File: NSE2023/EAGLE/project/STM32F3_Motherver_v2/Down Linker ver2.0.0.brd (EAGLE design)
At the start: 35.5 x 45.4 mm, 27 parts

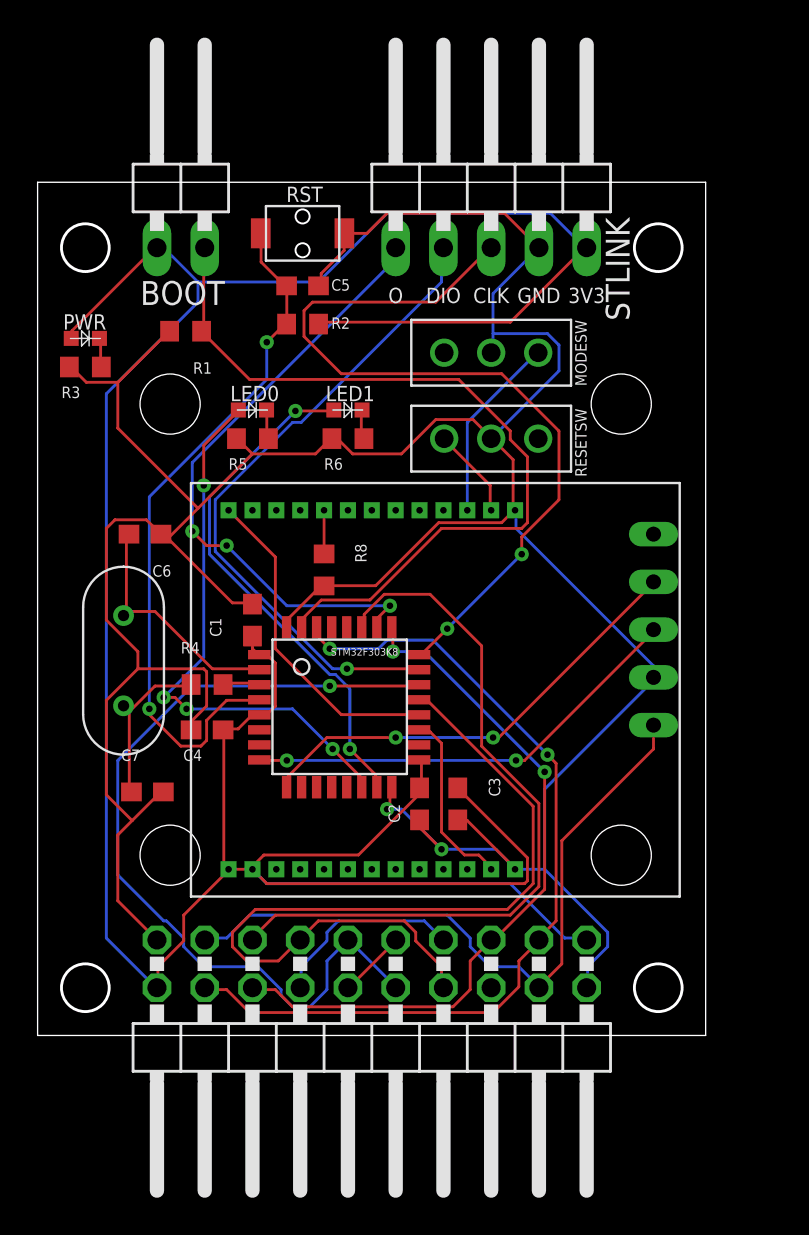
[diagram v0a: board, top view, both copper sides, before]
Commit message: create final board NSE2023
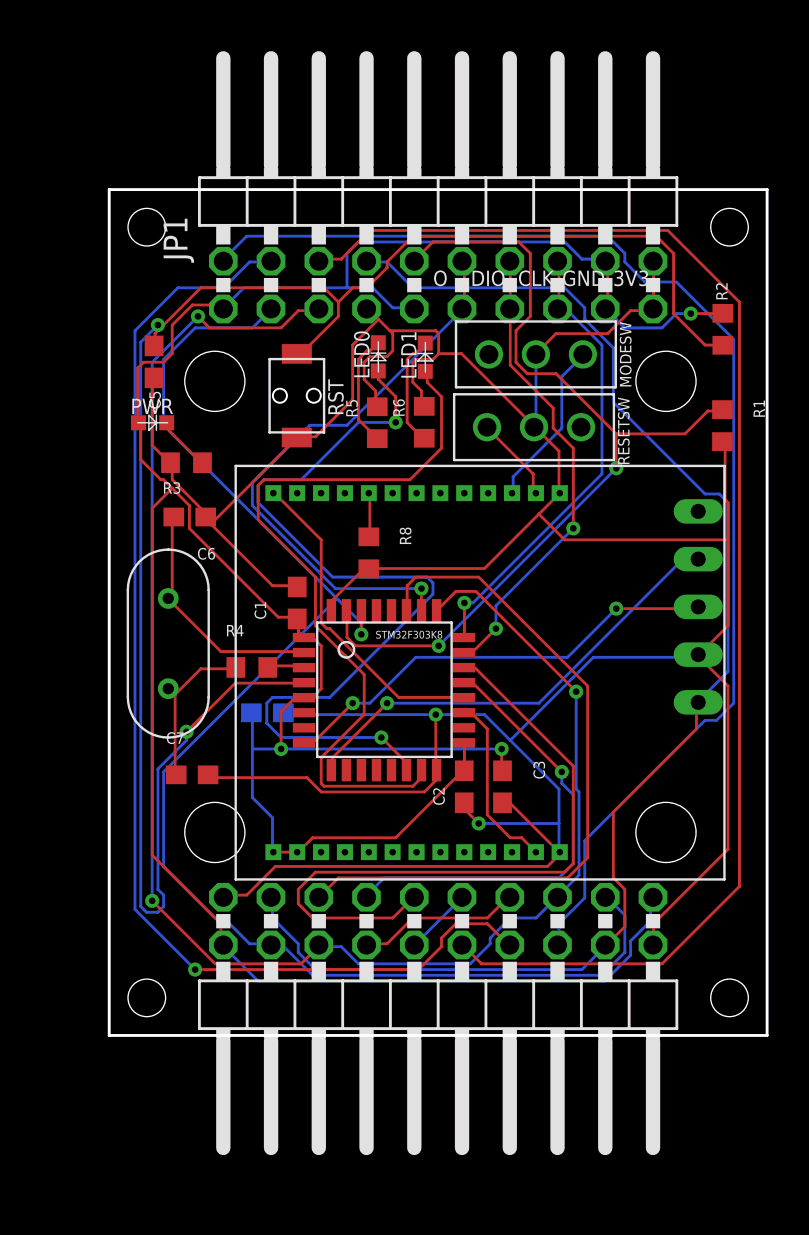
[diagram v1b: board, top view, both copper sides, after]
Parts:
- removed BOOT: (no value), pinhead:1X02/90
- removed STLINK: (no value), pinhead:1X05/90
- added JP1: (no value), pinhead:2X10/90
- added U$4: F.T.E.LOGO, logo:LOGO
- moved R1 29.0 mm to (32.6, 32.4), turned to 270 degrees
- moved R2 22.4 mm to (32.6, 37.6), turned to 90 degrees
- moved C5 8.87 mm to (2.39, 35.8), turned to 270 degrees
- moved RST 8.64 mm to (9.98, 34.0), turned to 0 degrees
- moved R3 7.41 mm to (4.11, 30.5)
- moved LED0 7.27 mm to (14.3, 36.1), turned to 90 degrees
- moved R5 6.69 mm to (14.3, 32.6), turned to 270 degrees
- moved PWR 5.74 mm to (2.31, 32.6)
- moved LED1 4.98 mm to (16.8, 36.1), turned to 90 degrees
- moved JP3 4.20 mm to (17.5, 1.00)
- moved R6 4.15 mm to (16.8, 32.6), turned to 270 degrees
- moved C4 3.33 mm to (8.41, 17.2), flipped to the bottom
- moved U$2 2.67 mm to (17.6, 22.8)
- moved R8 2.55 mm to (13.8, 25.7)
- moved U$1 2.55 mm to (11.0, 14.1)
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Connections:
- new net FPRAW: JP1.6, JP3.10
- new net SW: JP1.4, JP3.8
- net +3V3: now also JP1.1, JP1.17, JP1.18, JP1.9; no longer BOOT.1, STLINK.5
- net +5V: now also JP1.8
- net BIT1: no longer JP3.10
- net BIT2: no longer JP3.8
- net BOOT0: now also JP1.10; no longer BOOT.2
- net GND: now also JP1.19, JP1.20, JP1.7; no longer STLINK.4
- net PWM: now also JP1.2
- net SCL: now also JP1.5
- net SDA: now also JP1.3
- net SWCLK: now also JP1.15, JP1.16; no longer STLINK.3
- net SWDIO: now also JP1.13, JP1.14; no longer STLINK.2
- net SWO: now also JP1.11, JP1.12; no longer STLINK.1
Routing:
- net FPRAW: track 0.00 -> 72.6 mm
- net PWM: track 0.00 -> 66.8 mm
- net SW: track 0.00 -> 62.5 mm, vias 0 -> 1
- net NRST: track 37.5 -> 92.5 mm
- net SCL: track 37.8 -> 86.2 mm, vias 2 -> 3
- net +5V: track 36.7 -> 74.2 mm
- net SDA: track 46.9 -> 76.1 mm, vias 2 -> 1
- net BIT2: track 45.2 -> 24.1 mm, vias 0 -> 1
- net GND: track 183.3 -> 202.8 mm
- net SWCLK: track 43.4 -> 24.7 mm, vias 2 -> 1
- net LED0: track 29.7 -> 45.4 mm, vias 4 -> 2
- net LED1: track 27.8 -> 40.1 mm, vias 2 -> 0
- net SWDIO: track 35.0 -> 24.9 mm, vias 1 -> 2
- net BIT1: track 45.4 -> 36.1 mm, vias 1 -> 0
- net +3V3: track 167.2 -> 159.5 mm, vias 0 -> 3
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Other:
- board size 35.5 x 45.4 mm -> 35 x 45 mm

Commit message: www
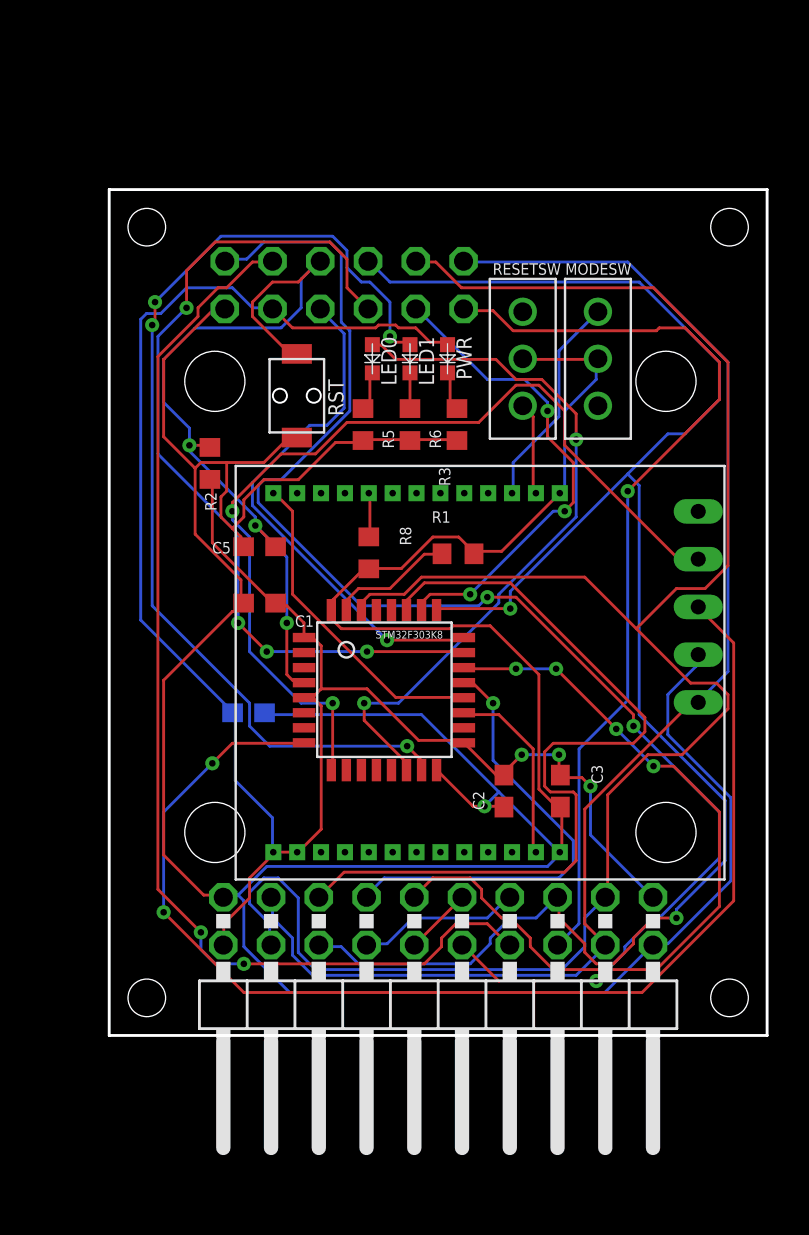
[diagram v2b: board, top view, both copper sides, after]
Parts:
- removed C6, C7: 30pF, rcl:C1608
- removed CRY1: (no value), Crystal:CRYSTAL
- removed JP1: (no value), pinhead:2X10/90
- removed R4: DNF, rcl:R0603
- removed U$4: F.T.E.LOGO, logo:LOGO
- added JP2: (no value), pinhead:2X06/90
- moved R2 28.2 mm to (5.36, 30.4), turned to 270 degrees
- moved PWR 16.1 mm to (18.0, 36.0), turned to 270 degrees
- moved R1 15.6 mm to (18.6, 25.6), turned to 0 degrees
- moved R3 14.5 mm to (18.5, 32.5), turned to 90 degrees
- moved C5 11.3 mm to (8.00, 26.0), turned to 180 degrees
- moved RESETSW 3.69 mm to (22.0, 36.0), turned to 270 degrees
- moved MODESW 3.31 mm to (26.0, 36.0), turned to 90 degrees
- moved C3 3.09 mm to (24.0, 13.0)
- moved C2 2.12 mm to (21.0, 13.0)
- moved C1 2.00 mm to (8.00, 23.0), turned to 180 degrees
- moved C4 1.00 mm to (7.41, 17.2)
- moved LED1 0.82 mm to (16.0, 36.0), turned to 270 degrees
- moved R6 0.77 mm to (16.0, 32.5), turned to 90 degrees
- moved R5 0.77 mm to (13.5, 32.5), turned to 90 degrees
- moved LED0 0.33 mm to (14.0, 36.0), turned to 270 degrees
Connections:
- removed net N$3: C7.1, CRY1.P$2, R4.1
- net +3V3: now also JP2.9; no longer JP1.1, JP1.17, JP1.18, JP1.9
- net +5V: now also JP2.2; no longer JP1.8
- net BOOT0: no longer JP1.10
- net FPRAW: now also JP2.12; no longer JP1.6
- net GND: now also JP2.11; no longer C6.2, C7.2, JP1.19, JP1.20, JP1.7
- net NRST: now also JP2.8
- net OSC_IN: no longer C6.1, CRY1.P$1
- net OSC_OUT: no longer R4.2
- net PWM: now also JP2.1; no longer JP1.2
- net SCL: now also JP2.6; no longer JP1.5
- net SDA: now also JP2.4; no longer JP1.3
- net SW: now also JP2.10; no longer JP1.4
- net SWCLK: now also JP2.7; no longer JP1.15, JP1.16
- net SWDIO: now also JP2.5; no longer JP1.13, JP1.14
- net SWO: now also JP2.3; no longer JP1.11, JP1.12
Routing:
- net +3V3: track 159.5 -> 107.5 mm
- net NRST: track 92.5 -> 43.2 mm, vias 2 -> 3
- net BOOT0: track 47.8 -> 6.63 mm, vias 2 -> 0
- net GPSRX: track 24.0 -> 64.9 mm
- net SDA: track 76.1 -> 102.3 mm, vias 1 -> 0
- net GPSTX: track 24.5 -> 49.7 mm, vias 1 -> 2
- net SWDIO: track 24.9 -> 46.5 mm, vias 2 -> 4
- net PWM: track 66.8 -> 49.5 mm, vias 0 -> 1
- net LED1: track 40.1 -> 54.2 mm, vias 0 -> 4
- net OSC_IN: track 12.9 -> 0.00 mm
- net N$3: track 9.14 -> 0.00 mm
- net SCL: track 86.2 -> 94.6 mm, vias 3 -> 2
- net LED0: track 45.4 -> 38.0 mm
- net FP_CHECKER: track 37.8 -> 44.8 mm
- net BIT1: track 36.1 -> 42.4 mm, vias 0 -> 4
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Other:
- board text removed: "3V3"
- board text removed: "CLK"
- board text removed: "DIO"
- board text removed: "GND"
- board text removed: "O"
